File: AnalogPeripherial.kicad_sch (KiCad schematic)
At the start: 24 parts, among them J1 SD_Card_Receptacle, U1 74HC7014, U2 LD1117S33TR_SOT223, U3 STM32F407VGTx, U4 TLV9061xDBV

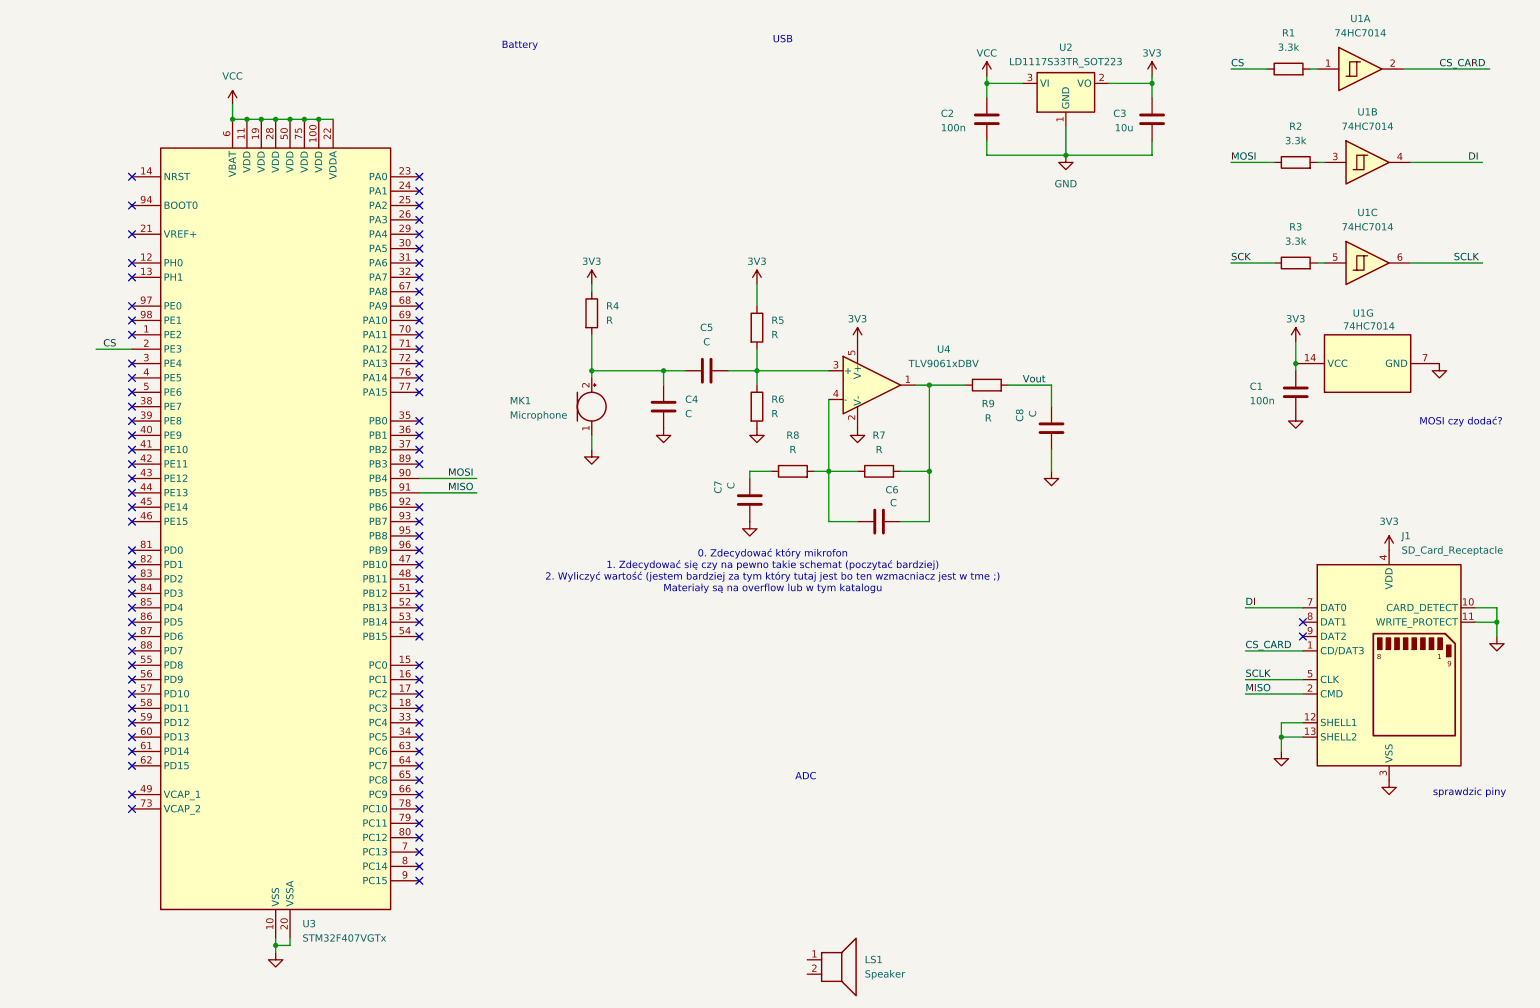
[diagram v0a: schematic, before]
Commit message: Almost finished schemat design
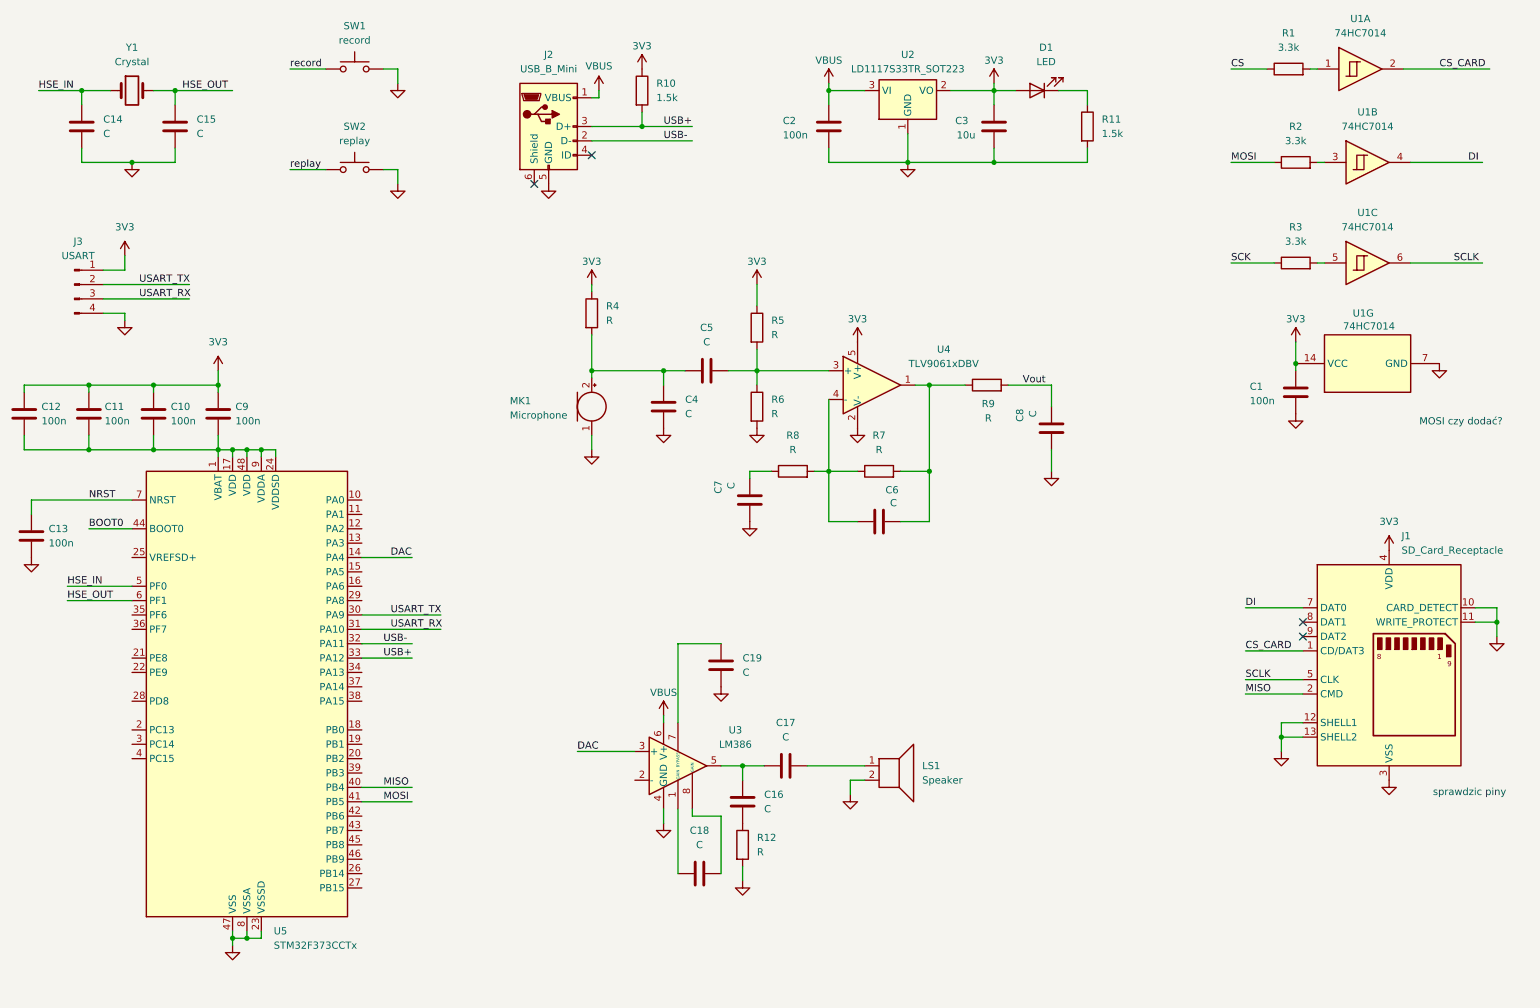
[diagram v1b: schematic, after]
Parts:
- removed U3: STM32F407VGTx, Package_QFP:LQFP-100_14x14mm_P0.5mm, symbol MCU_ST_STM32F4:STM32F407VGTx
- added C10, C11, C12, C13, C9: 100n, symbol Device:C
- added C14, C15, C16, C17, C18, C19: C, symbol Device:C
- added D1: LED, symbol Device:LED
- added J2: USB_B_Mini, symbol Connector:USB_B_Mini
- added J3: USART, symbol Connector:Conn_01x04_Pin
- added R10, R11: 1.5k, symbol Device:R
- added R12: R, symbol Device:R
- added SW1: record, symbol Switch:SW_Push
- added SW2: replay, symbol Switch:SW_Push
- added U3: LM386, symbol Amplifier_Audio:LM386
- added U5: STM32F373CCTx, Package_QFP:LQFP-48_7x7mm_P0.5mm, symbol MCU_ST_STM32F3:STM32F373CCTx
- added Y1: Crystal, symbol Device:Crystal
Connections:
- net 3V3: now also C10.1, C11.1, C12.1, C9.1, D1.2 (A), J3.1 (Pin_1), R10.1
- net GND: now also LS1.2, C13.2, C14.2, C15.2, C19.1, J2.5 (GND), J3.4 (Pin_4), R11.2, R12.2, SW1.2, SW2.2, U3.4 (GND), U5.23 (VSSSD), U5.47 (VSS), U5.8 (VSSA)
- net MISO: now also U5.40 (PB4)
- net MOSI: now also U5.41 (PB5)
- net at LS1.1: now also C17.2
- net VCC renamed VBUS
- net VBUS: now also J2.1 (VBUS), U3.6 (V+)
- new net: C16.2, R12.1
- new net: C18.1, U3.1 (GAIN)
- new net: C18.2, U3.8 (GAIN)
- new net: C16.1, C17.1, U3.5
- new net: C19.2, U3.7 (BYPASS)
- new net: C10.2, C11.2, C12.2, C9.2, U5.1 (VBAT), U5.17 (VDD), U5.24 (VDDSD), U5.48 (VDD), U5.9 (VDDA)
- new net: D1.1 (K), R11.1
- new net BOOT0: U5.44 (BOOT0)
- new net DAC: U3.3 (+), U5.14 (PA4)
- new net HSE_IN: C14.1, U5.5 (PF0), Y1.1
- new net HSE_OUT: C15.1, U5.6 (PF1), Y1.2
- new net NRST: C13.1, U5.7 (NRST)
- new net USART_RX: J3.3 (Pin_3), U5.31 (PA10)
- new net USART_TX: J3.2 (Pin_2), U5.30 (PA9)
- new net USB+: J2.3 (D+), R10.2, U5.33 (PA12)
- new net USB-: J2.2 (D-), U5.32 (PA11)
- new net record: SW1.1
- new net replay: SW2.1
- no-connect marks 86 -> 4
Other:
- note removed: "0. Zdecydować który mikrofon 1. Zdecydować się czy na pewno takie schemat (poczytać bardziej) 2. Wyliczyć wartość (jestem bardziej za tym który tutaj jest bo ten wzmacniacz jest w tme ;) Materiały są na overflow lub w tym katalogu"
- note removed: "ADC"
- note removed: "Battery"
- note removed: "USB"
- moved on the sheet: C2, C3, LS1, U2
